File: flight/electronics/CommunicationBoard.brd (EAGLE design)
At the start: 90 x 90 mm, 11 parts, among them J1 CONUFL001-SMD-T, X1 JST-XH-02-PIN

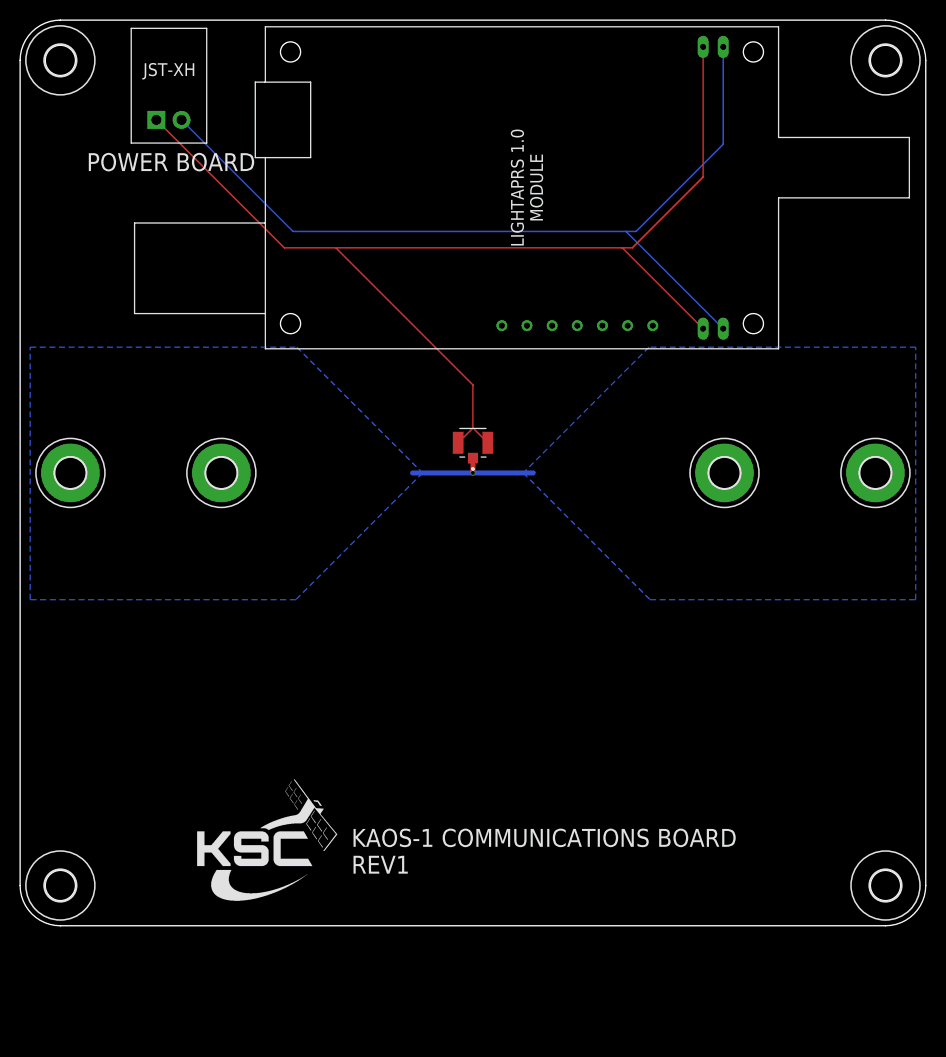
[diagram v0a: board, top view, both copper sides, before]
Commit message: final touches
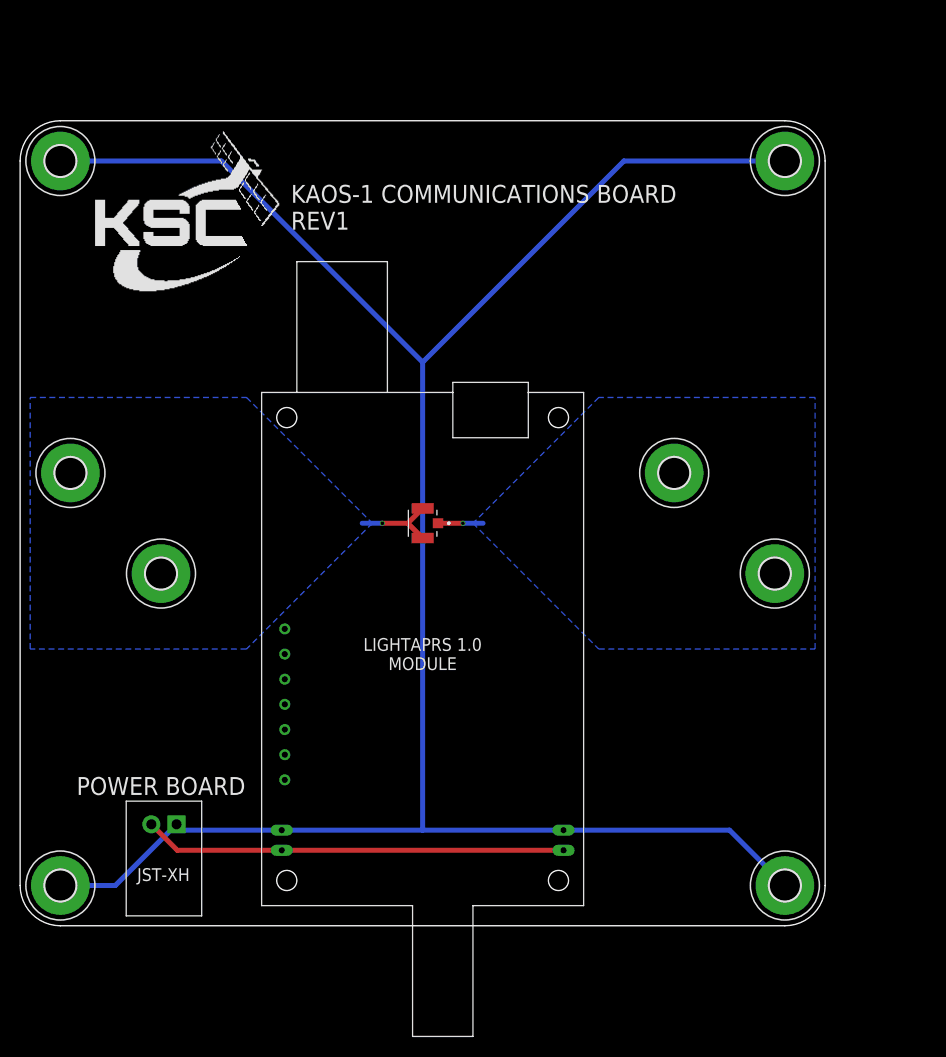
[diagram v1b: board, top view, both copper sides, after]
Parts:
- removed U$2, U$3, U$4, U$5: (no value), holes:3,0
- added H5, H6, H7, H8: MOUNT-PAD-ROUND3.0, holes:3,0-PAD
- moved X1 70.0 mm to (15.5, 10.1), turned to 180 degrees
- moved U$1 47.5 mm to (40.0, 27.0), turned to 180 degrees
- moved H1 14.1 mm to (75.0, 35.0)
- moved H3 11.7 mm to (14.0, 35.0)
- moved J1 9.43 mm to (40.0, 40.0), turned to 90 degrees
- moved H2 5.00 mm to (65.0, 45.0)
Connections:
- removed net SIG: H1.B3,0, H2.B3,0, H3.B3,0, H4.B3,0, J1.1
- new net SIG+: H1.B3,0, H2.B3,0, J1.1
- new net SIG-: H3.B3,0, H4.B3,0, J1.2, J1.3
- net GND: now also H5.B3,0, H6.B3,0, H7.B3,0, H8.B3,0; no longer J1.2, J1.3
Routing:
- net GND: track 114.5 -> 212.1 mm
- net VBAT: track 85.3 -> 42.0 mm
- net SIG: track 13.5 -> 0.00 mm, vias 1 -> 0
- net SIG-: track 0.00 -> 8.70 mm, vias 0 -> 1
- net SIG+: track 0.00 -> 4.48 mm, vias 0 -> 1
- added copper zone on layer 16, net SIG+
- added copper zone on layer 16, net SIG-
- removed copper zone on layer 16, net SIG
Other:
- board size 90 x 90 mm -> 80 x 80 mm
- board text removed: "/home/webbgamers/Downloads/KSC-logoPrimary.bmp"

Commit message: final board tweaks
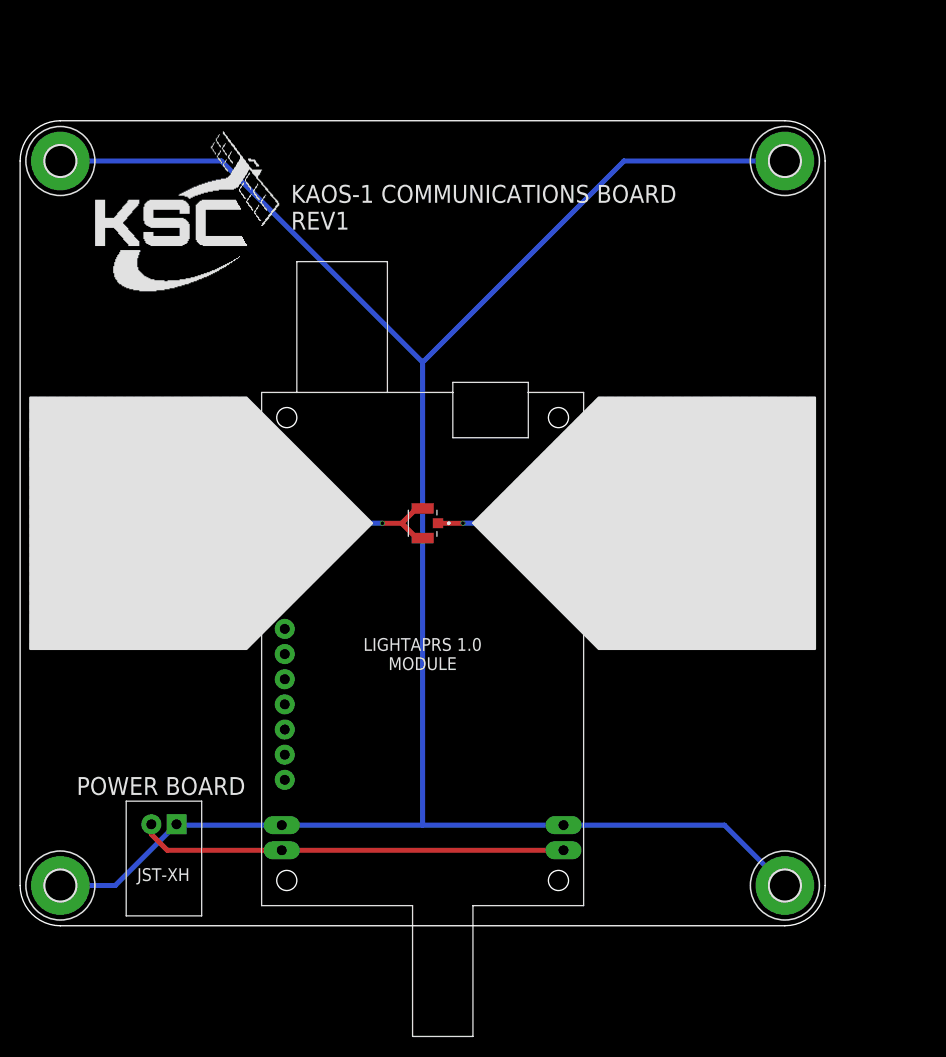
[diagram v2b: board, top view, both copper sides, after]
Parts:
- X1: device Rembrandt Electronics - JST XH Connectors v1-0:JST-XH_S2B -> JST-XH Connectors:JST-XH_S2B
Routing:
- net SIG-: track 8.70 -> 9.30 mm
- net VBAT: track 42.0 -> 42.6 mm
- net GND: track 212.1 -> 211.6 mm
